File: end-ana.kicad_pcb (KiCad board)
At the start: 2 copper layers, 160 x 80 mm, 10 parts

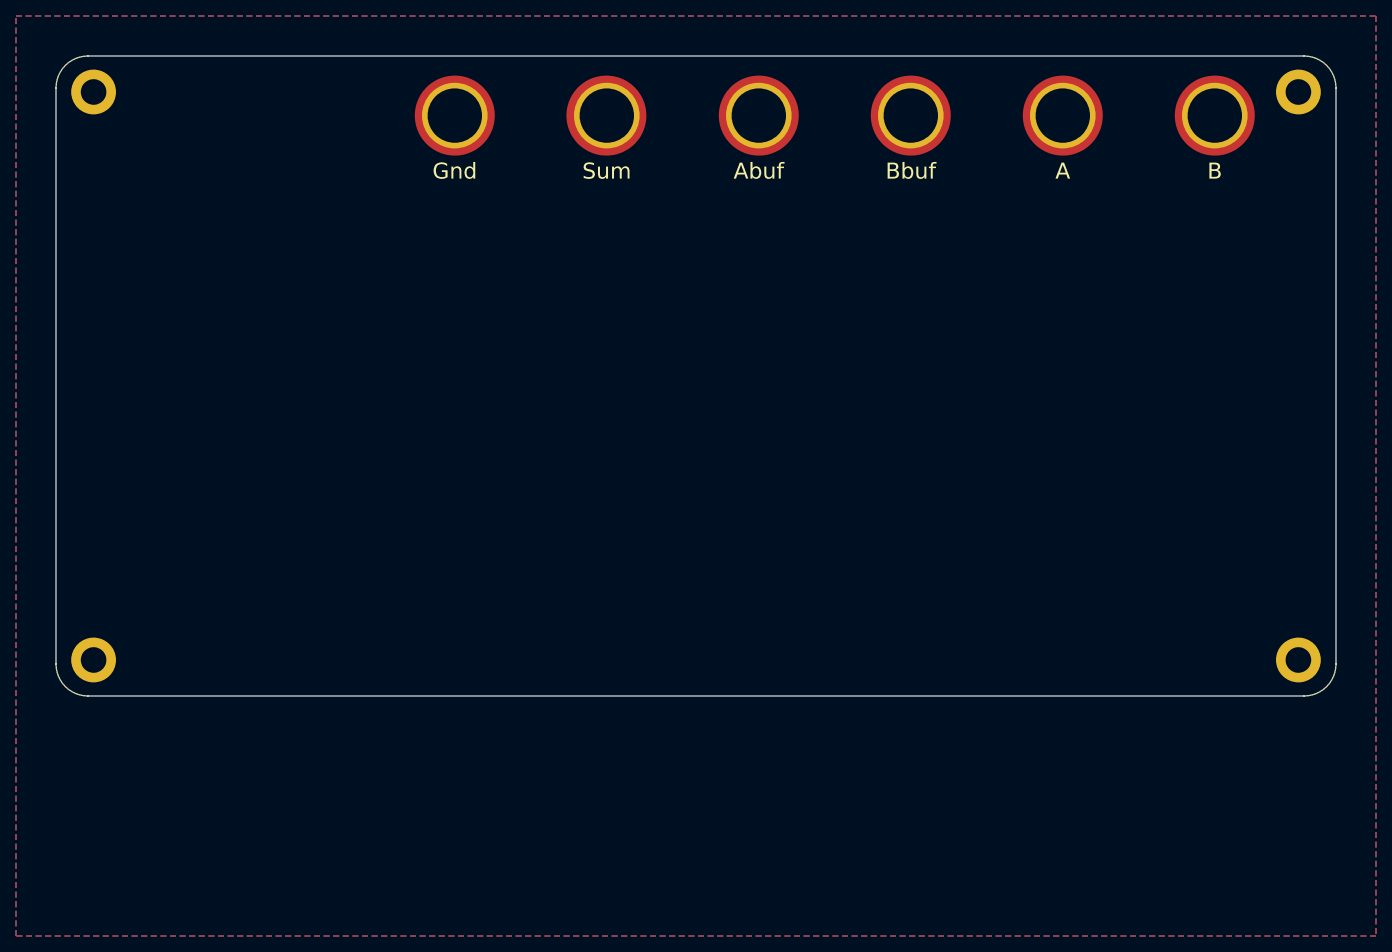
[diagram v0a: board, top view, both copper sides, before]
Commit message: Contact pads.  Shuffle the big cap.
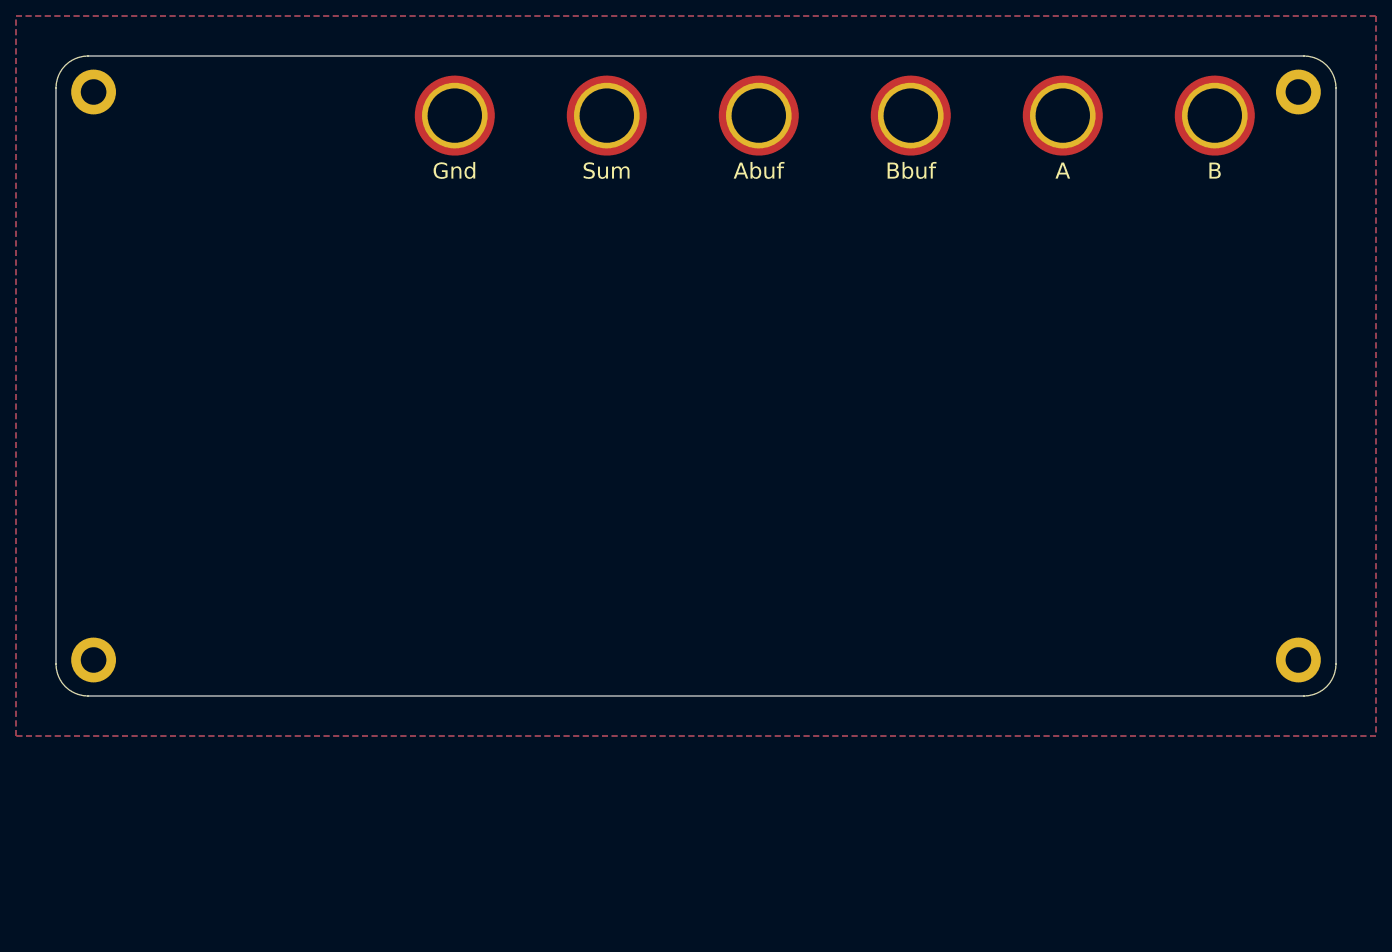
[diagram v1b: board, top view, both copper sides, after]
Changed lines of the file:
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@@
+			(thermal_bridge_angle 90)
+		)
+		(pad "1" smd circle
+			(at 0 0)
+			(size 10 10)
+			(layers "F.Cu" "F.Mask")
+			(net 6 "/Gnd")
+			(pinfunction "1")
+			(pintype "input")
 			(thermal_bridge_angle 90)
 		)
@@
 			(thermal_bridge_angle 90)
 		)
+		(pad "1" smd circle
+			(at 0 0)
+			(size 10 10)
+			(layers "F.Cu" "F.Mask")
+			(net 7 "/Bbuf")
+			(pinfunction "1")
+			(pintype "input")
+			(thermal_bridge_angle 90)
+		)
 		(embedded_fonts no)
 	)
@@
 			(thermal_bridge_angle 90)
 		)
+		(pad "1" smd circle
+			(at 0 0)
+			(size 10 10)
+			(layers "F.Cu" "F.Mask")
+			(net 4 "/Abuf")
+			(pinfunction "1")
+			(pintype "input")
+			(thermal_bridge_angle 90)
+		)
 		(embedded_fonts no)
 	)
@@
 			(thermal_bridge_angle 90)
 		)
+		(pad "1" smd circle
+			(at 0 0)
+			(size 10 10)
+			(layers "F.Cu" "F.Mask")
+			(net 2 "/A")
+			(pinfunction "1")
+			(pintype "input")
+			(thermal_bridge_angle 90)
+		)
 		(embedded_fonts no)
 	)
@@
 			(thermal_bridge_angle 90)
 		)
+		(pad "1" smd circle
+			(at 0 0)
+			(size 10 10)
+			(layers "F.Cu" "F.Mask")
+			(net 3 "/B")
+			(pinfunction "1")
+			(pintype "input")
+			(thermal_bridge_angle 90)
+		)
 		(embedded_fonts no)
 	)
@@
 			(thermal_bridge_angle 90)
 		)
+		(pad "1" smd circle
+			(at 0 0)
+			(size 10 10)
+			(layers "F.Cu" "F.Mask")
+			(net 5 "/Sum")
+			(pinfunction "1")
+			(pintype "input")
+			(thermal_bridge_angle 90)
+		)
 		(embedded_fonts no)
 	)
-	(gr_circle
-		(center 119.85 67.45)
-		(end 124.85 67.45)
+	(gr_rect
+		(start 128 72)
+		(end 132 74)
 		(stroke
 			(width 0)
@@
 		)
 		(fill yes)
-		(layer "F.Cu")
-		(net 6)
-	)
-	(gr_circle
-		(center 214.85 67.45)
-		(end 219.85 67.45)
-		(stroke
-			(width 0)
-			(type default)
-		)
-		(fill yes)
-		(layer "F.Cu")
-		(net 3)
-	)
-	(gr_circle
-		(center 176.85 67.45)
-		(end 181.85 67.45)
-		(stroke
-			(width 0)
-			(type default)
-		)
-		(fill yes)
-		(layer "F.Cu")
-		(net 7)
-	)
-	(gr_circle
-		(center 195.85 67.45)
-		(end 200.85 67.45)
-		(stroke
-			(width 0)
-			(type default)
-		)
-		(fill yes)
-		(layer "F.Cu")
-		(net 2)
-	)
-	(gr_circle
-		(center 138.8 67.45)
-		(end 143.8 67.45)
-		(stroke
-			(width 0)
-			(type default)
-		)
-		(fill yes)
-		(layer "F.Cu")
-		(net 5)
-	)
-	(gr_circle
-		(center 157.85 67.45)
-		(end 162.85 67.45)
-		(stroke
-			(width 0)
-			(type default)
-		)
-		(fill yes)
-		(layer "F.Cu")
-		(net 4)
+		(layer "B.Mask")
 	)
 	(gr_arc
@@
 		(net 1)
 		(net_name "GNDPWR")
-		(locked yes)
 		(layers "F.Cu" "B.Cu")
 		(name "Gnd")
@@
 		(polygon
 			(pts
-				(xy 65 55) (xy 235 55) (xy 235 170) (xy 65 170)
+				(xy 65 55) (xy 235 55) (xy 235 145) (xy 65 145)
 			)
 		)
@@
 		(net 0)
 		(net_name "")
+		(locked yes)
 		(layer "B.Mask")
 		(name "Earth")
